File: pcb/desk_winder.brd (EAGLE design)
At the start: 161.3 x 100 mm, 14 parts, among them IC1 TINY13-20PU, IC2 7805L, J1 22-27-2041-04, X1 22-23-2021, X2 22-23-2031

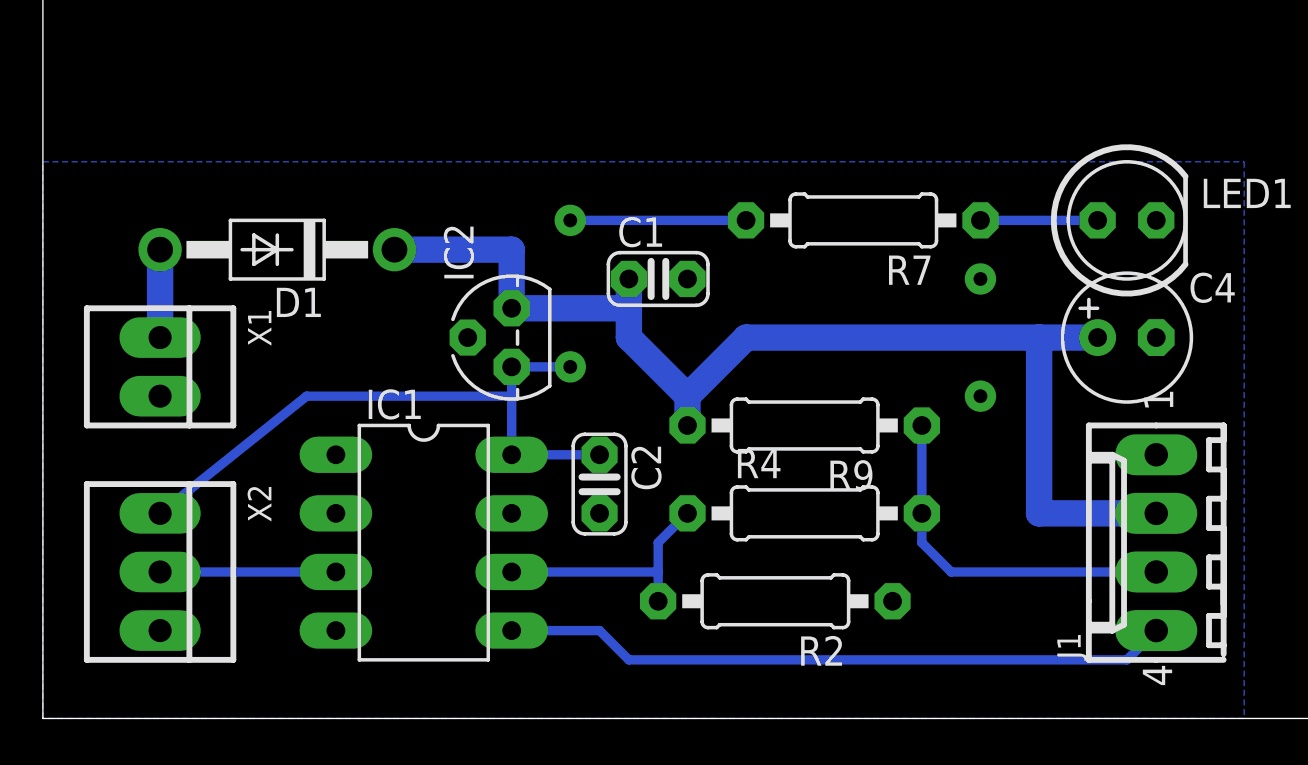
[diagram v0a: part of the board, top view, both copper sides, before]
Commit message: pcb
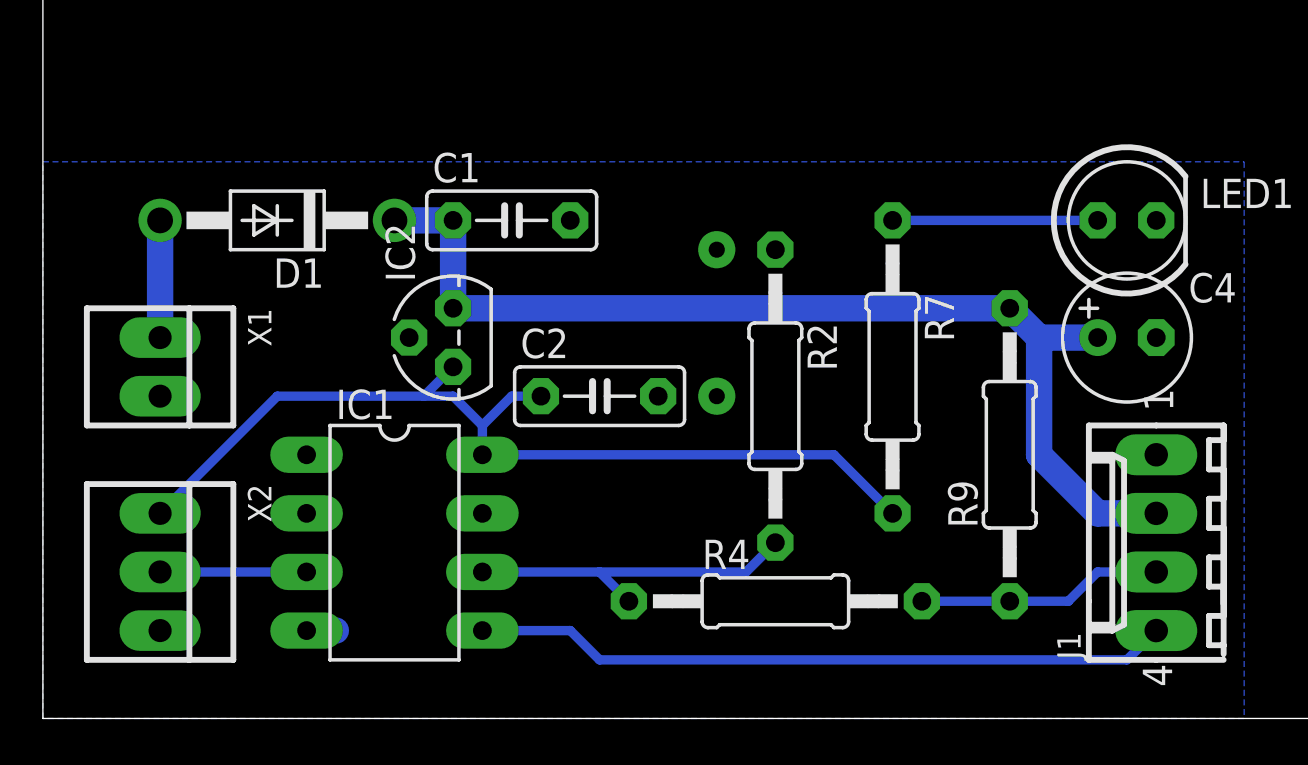
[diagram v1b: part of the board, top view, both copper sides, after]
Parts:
- C1, C2: device rcl:C025-024X044 -> rcl:C050-025X075
- R2: value 4.7k -> 8.2k; device resistor:0207/10 -> resistor:0207/12
- R4, R7, R9: device resistor:0207/10 -> resistor:0207/12
- moved R9 8.98 mm to (40.6, 11.4), turned to 90 degrees
- moved R2 8.89 mm to (30.5, 14.0), turned to 270 degrees
- moved C1 6.84 mm to (19.1, 21.6)
- moved R7 6.48 mm to (35.6, 15.2), turned to 270 degrees
- moved R4 4.02 mm to (30.5, 5.08)
- moved C2 3.81 mm to (22.9, 14.0), turned to 0 degrees
- moved IC2 2.54 mm to (16.5, 16.5)
- moved D1 1.27 mm to (8.89, 21.6)
- moved IC1 1.27 mm to (14.0, 7.62)
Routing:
- net VCC: track 34.8 -> 41.6 mm
- net +12V: track 51.6 -> 46.0 mm
- net SENSE: track 15.8 -> 10.7 mm
- net TACH_IN: track 10.7 -> 15.0 mm
- net N$1: track 5.08 -> 8.89 mm
- net VDD: track 3.81 -> 5.08 mm
- net POTZ: track 7.62 -> 6.35 mm
- net CTRL: track 29.0 -> 30.3 mm
- net GND: track 0.00 -> 1.27 mm
